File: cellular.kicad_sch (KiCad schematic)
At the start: 24 parts, among them J4 SIM_Card, Q2 BC847, U3 A7672SA__LASE_, U5 SMF15CT1G

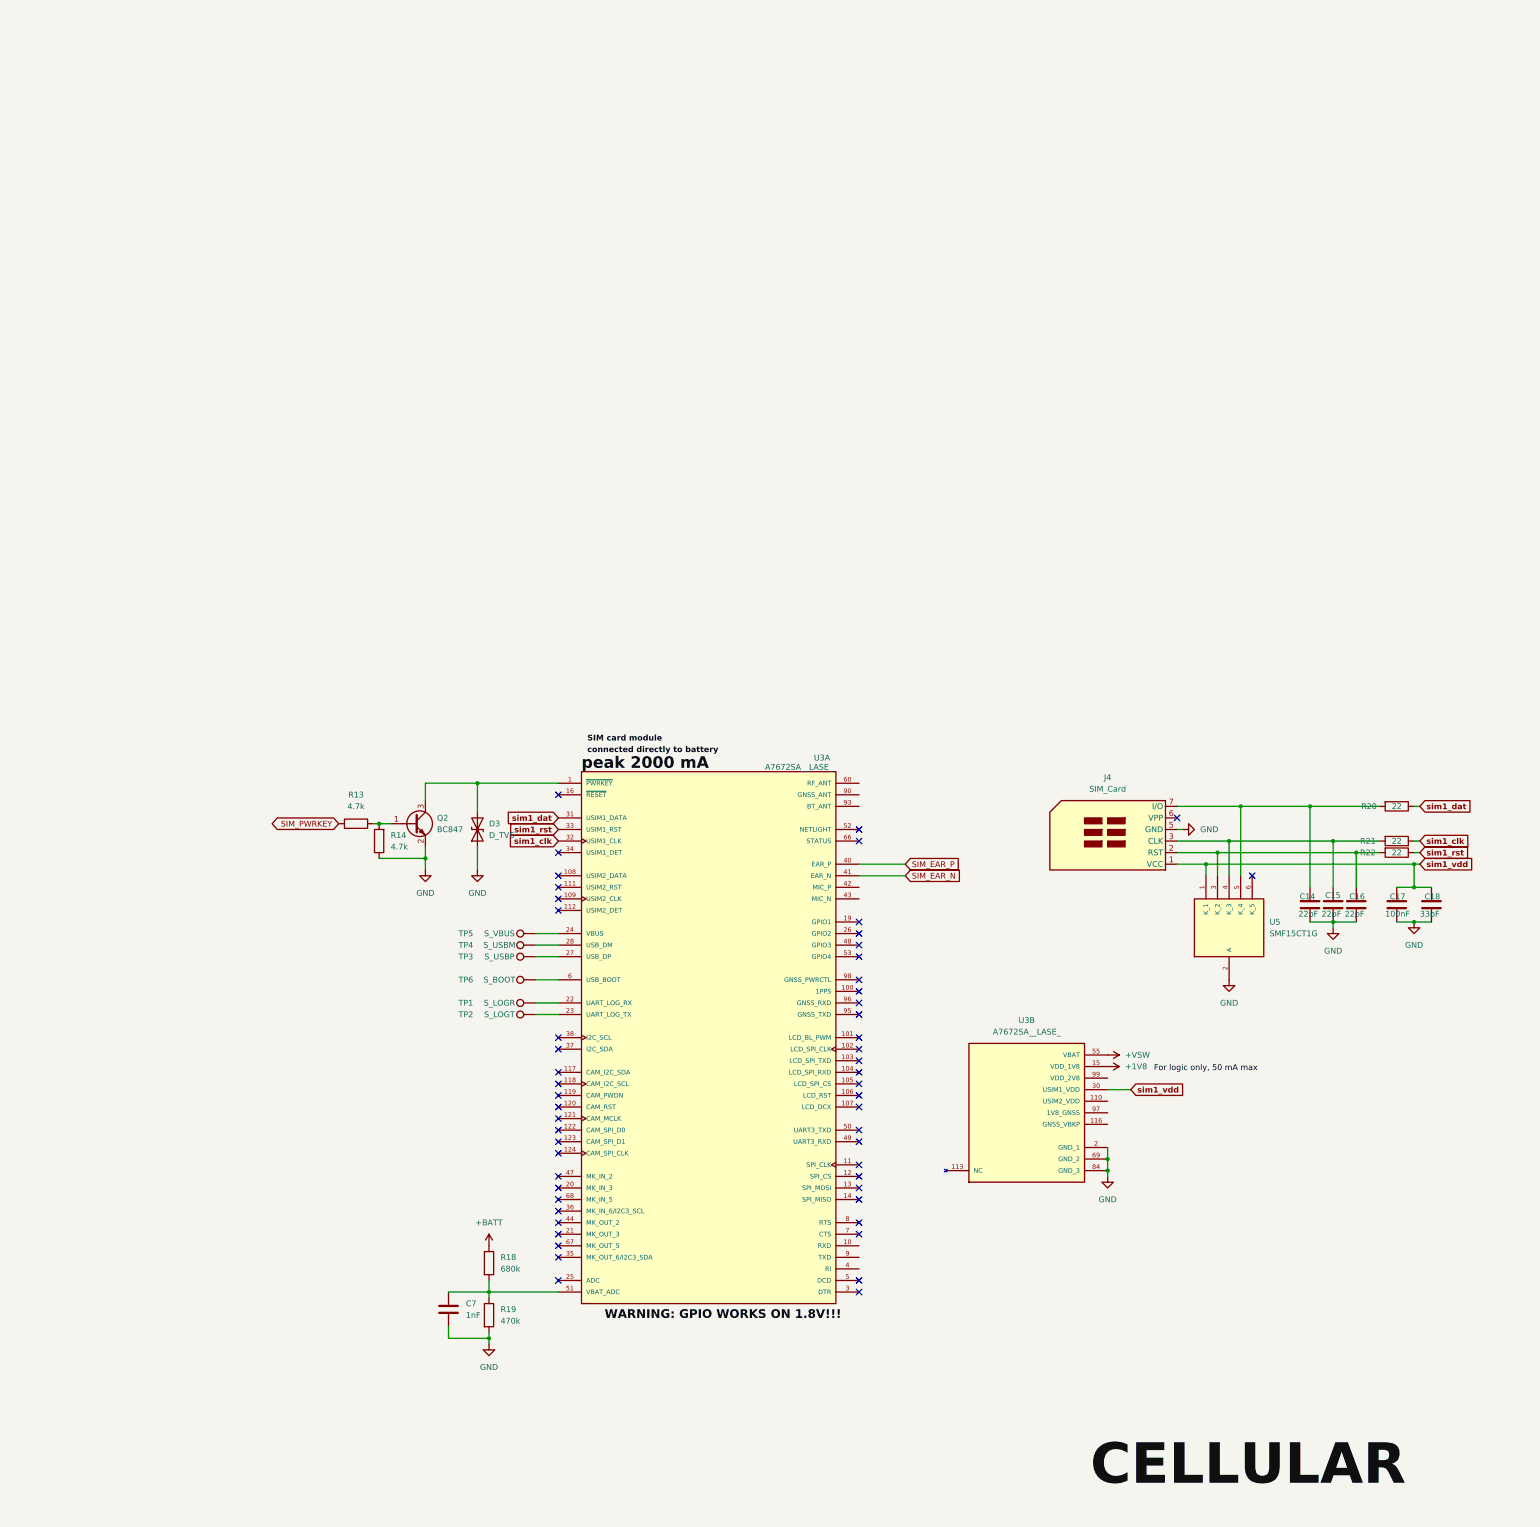
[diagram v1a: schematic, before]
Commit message: SCHEMATIC
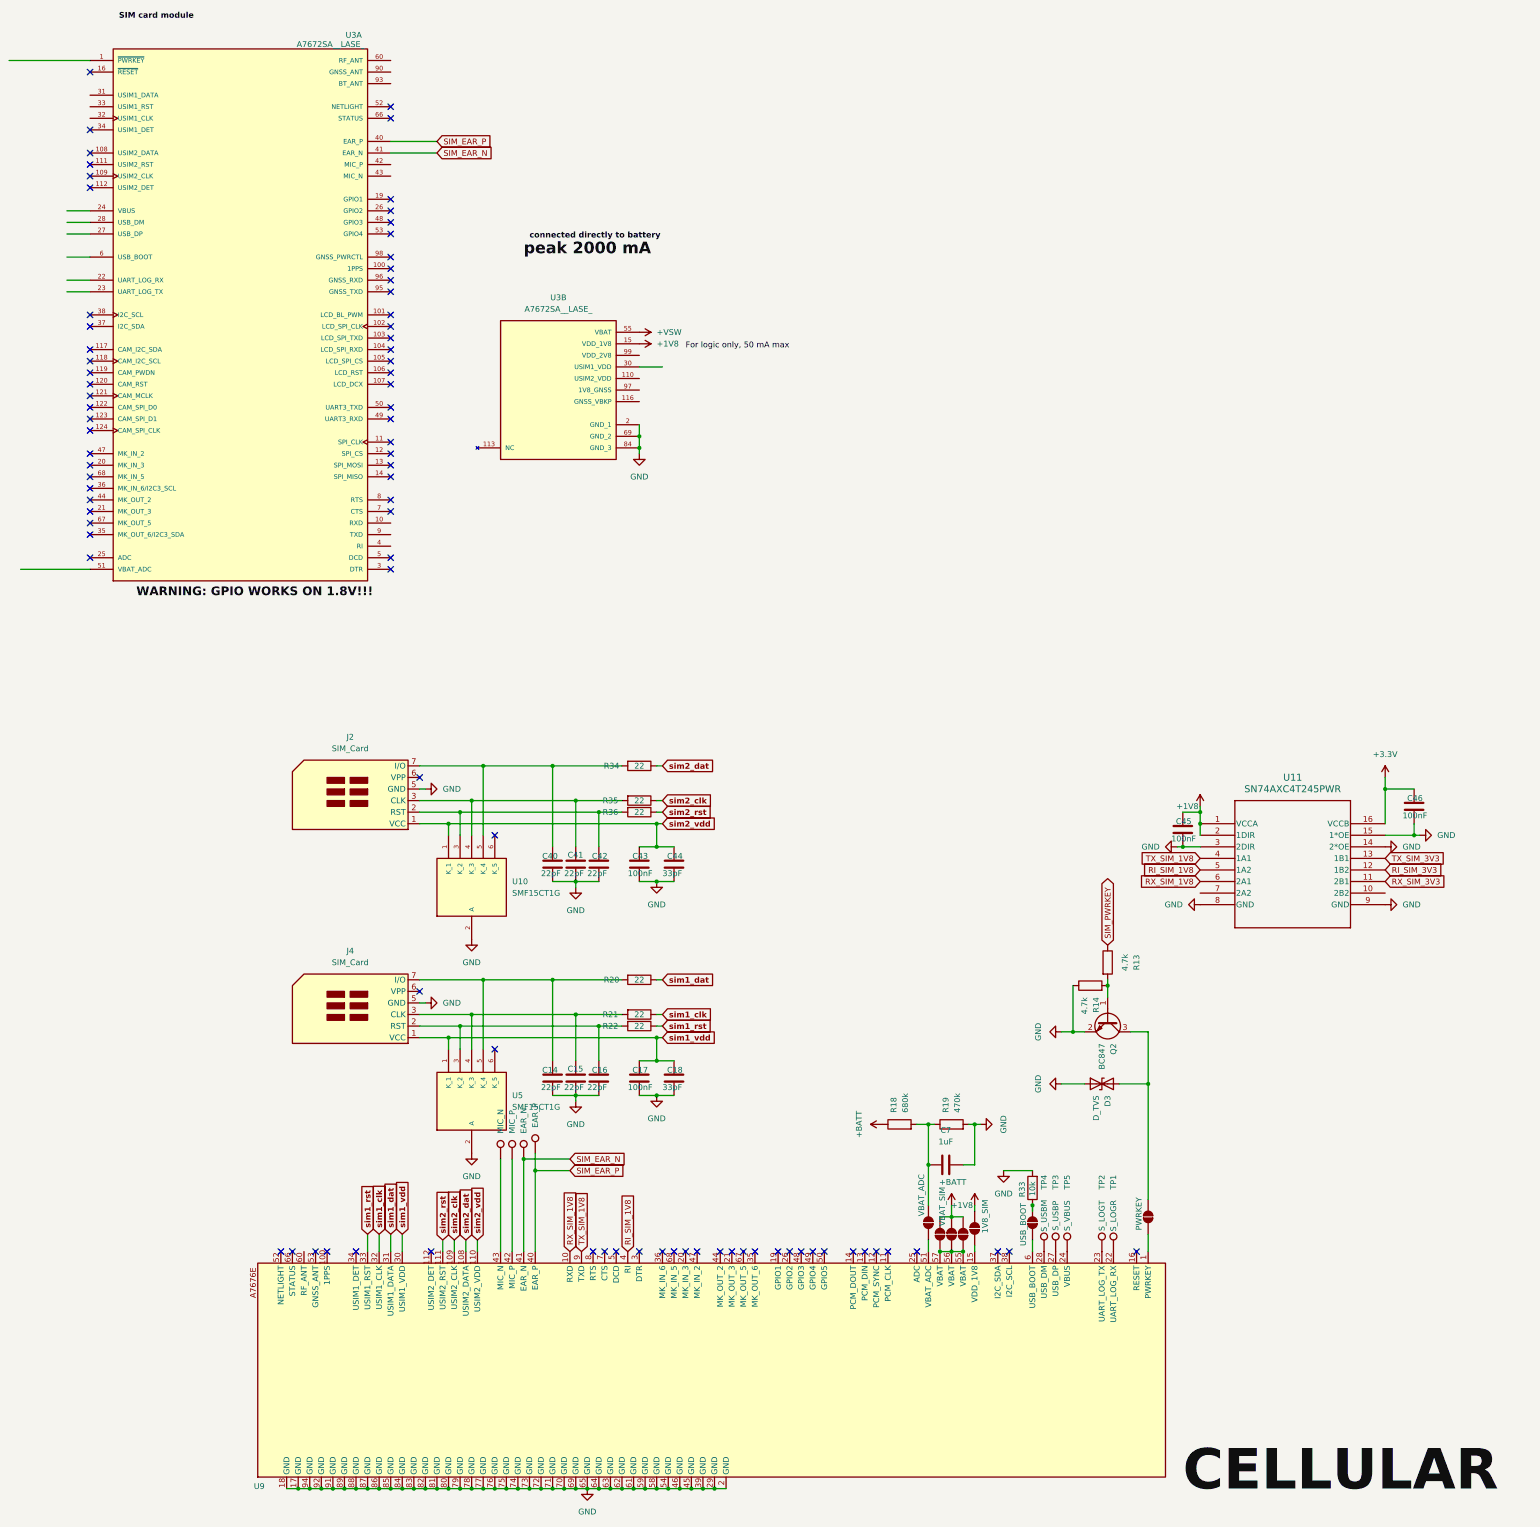
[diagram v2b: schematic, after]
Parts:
- removed TP6: S_BOOT, symbol Connector:TestPoint
- added 1V8_SIM, PWRKEY, USB_BOOT, VBAT_ADC, VBAT_SIM, VBAT_SIM1, VBAT_SIM2: SolderJumper_2_Open, Jumper:SolderJumper-2_P1.3mm_Open_Pad1.0x1.5mm, symbol Jumper:SolderJumper_2_Open
- added C40, C41, C42: 22pF, symbol Device:C
- added C43, C45, C46: 100nF, symbol Device:C
- added C44: 33pF, symbol Device:C
- added EAR_N, EAR_P, MIC_N, MIC_P: TestPoint, symbol Connector:TestPoint
- added J2: SIM_Card, symbol Connector:SIM_Card
- added R33: 10k, symbol Device:R
- added R34, R35, R36: 22, symbol Device:R
- added U10: SMF15CT1G, SMF15CT1G:SOT65P210X110-6N, symbol SMF15CT1G:SMF15CT1G
- added U11: SN74AXC4T245PWR, TSSOP16_PW_TEX, symbol SN74AXC4T245PWR:SN74AXC4T245PWR
- added U9: ~, symbol A7676E:A7676E
- C7: value 1nF -> 1uF
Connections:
- net +1V8: now also 1V8_SIM.2 (B), C45.1, U11.1 (VCCA), U11.2 (1DIR)
- net +BATT: now also VBAT_SIM.2 (B), VBAT_SIM1.2 (B), VBAT_SIM2.2 (B)
- net GND: now also C40.2, C41.2, C42.2, C43.2, C44.2, C45.2, C46.2, J2.5 (GND), R33.2, U10.2 (A), U11.14 (2*OE), U11.15 (1*OE), U11.3 (2DIR), U11.8 (GND), U11.9 (GND), U9.17 (GND), U9.18 (GND), U9.2 (GND), U9.29 (GND), U9.39 (GND), U9.45 (GND), U9.46 (GND), U9.54 (GND), U9.58 (GND), U9.59 (GND), U9.61 (GND), U9.62 (GND), U9.63 (GND), U9.64 (GND), U9.65 (GND), U9.69 (GND), U9.70 (GND), U9.71 (GND), U9.72 (GND), U9.73 (GND), U9.74 (GND), U9.75 (GND), U9.76 (GND), U9.77 (GND), U9.78 (GND), U9.79 (GND), U9.80 (GND), U9.81 (GND), U9.82 (GND), U9.83 (GND), U9.84 (GND), U9.85 (GND), U9.86 (GND), U9.87 (GND), U9.88 (GND), U9.89 (GND), U9.91 (GND), U9.92 (GND), U9.94 (GND)
- net SIM_EAR_N: now also EAR_N.1, U9.41 (EAR_N)
- net SIM_EAR_P: now also EAR_P.1, U9.40 (EAR_P)
- net sim1_clk: now also U9.32 (USIM1_CLK); no longer U3.32 (USIM1_CLK)
- net sim1_dat: now also U9.31 (USIM1_DATA); no longer U3.31 (USIM1_DATA)
- net sim1_rst: now also U9.33 (USIM1_RST); no longer U3.33 (USIM1_RST)
- net sim1_vdd: now also U9.30 (USIM1_VDD); no longer U3.30 (USIM1_VDD)
- net at TP1.1: now also U9.22 (UART_LOG_RX); no longer U3.22 (UART_LOG_RX)
- net at C7.1, R18.2, R19.1: now also VBAT_ADC.2 (B); no longer U3.51 (VBAT_ADC)
- net at TP3.1: now also U9.27 (USB_DP); no longer U3.27 (USB_DP)
- net at TP2.1: now also U9.23 (UART_LOG_TX); no longer U3.23 (UART_LOG_TX)
- net at TP5.1: now also U9.24 (VBUS); no longer U3.24 (VBUS)
- net at D3.2 (A2), Q2.3 (C): now also PWRKEY.2 (B); no longer U3.1 (~{PWRKEY})
- net at TP4.1: now also U9.28 (USB_DM); no longer U3.28 (USB_DM)
- new net: C42.1, J2.2 (RST), R36.2, U10.3 (K_2)
- new net: C41.1, J2.3 (CLK), R35.2, U10.4 (K_3)
- new net: C40.1, J2.7 (I/O), R34.2, U10.5 (K_4)
- new net: 1V8_SIM.1 (A), U9.15 (VDD_1V8)
- new net: U9.51 (VBAT_ADC), VBAT_ADC.1 (A)
- new net: U9.55 (VBAT), U9.56 (VBAT), U9.57 (VBAT), VBAT_SIM.1 (A), VBAT_SIM1.1 (A), VBAT_SIM2.1 (A)
- new net: PWRKEY.1 (A), U9.1 (PWRKEY)
- new net: MIC_P.1, U9.42 (MIC_P)
- new net: MIC_N.1, U9.43 (MIC_N)
- new net: U9.6 (USB_BOOT), USB_BOOT.1 (A)
- new net: R33.1, USB_BOOT.2 (B)
- new net +3.3V: C46.1, U11.16 (VCCB)
- new net RI_SIM_1V8: U11.5 (1A2), U9.4 (RI)
- new net RI_SIM_3V3: U11.12 (1B2)
- new net RX_SIM_1V8: U11.6 (2A1), U9.10 (RXD)
- new net RX_SIM_3V3: U11.11 (2B1)
- new net TX_SIM_1V8: U11.4 (1A1), U9.9 (TXD)
- new net TX_SIM_3V3: U11.13 (1B1)
- new net sim2_clk: R35.1, U9.109 (USIM2_CLK)
- new net sim2_dat: R34.1, U9.108 (USIM2_DATA)
- new net sim2_rst: R36.1, U9.111 (USIM2_RST)
- new net sim2_vdd: C43.1, C44.1, J2.1 (VCC), U10.1 (K_1), U9.110 (USIM2_VDD)
- no-connect marks 54 -> 87
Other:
- moved on the sheet: C14, C15, C16, C17, C18, C7, D3, J4, Q2, R13, R14, R18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
